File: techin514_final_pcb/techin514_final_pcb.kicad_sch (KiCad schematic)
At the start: 6 parts, among them M1 Motor_Servo, U1 ESP32-C3-DevKitM-1, U2 HC-SR04, U3 HC-SR04, U4 ESP32-C3-DevKitM-1

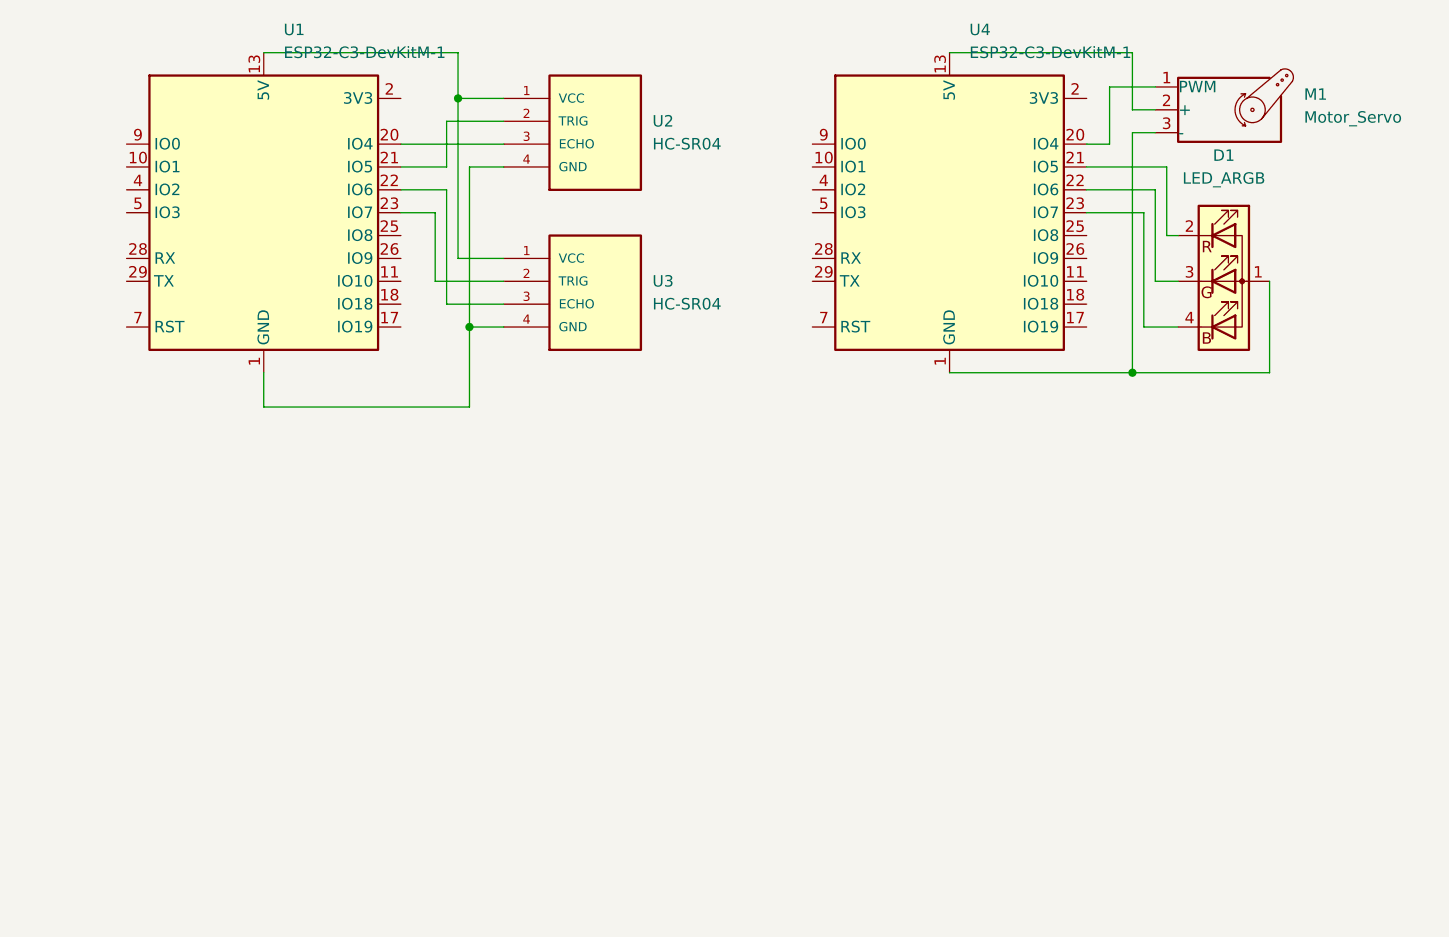
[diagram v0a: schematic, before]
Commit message: Datasheet updated
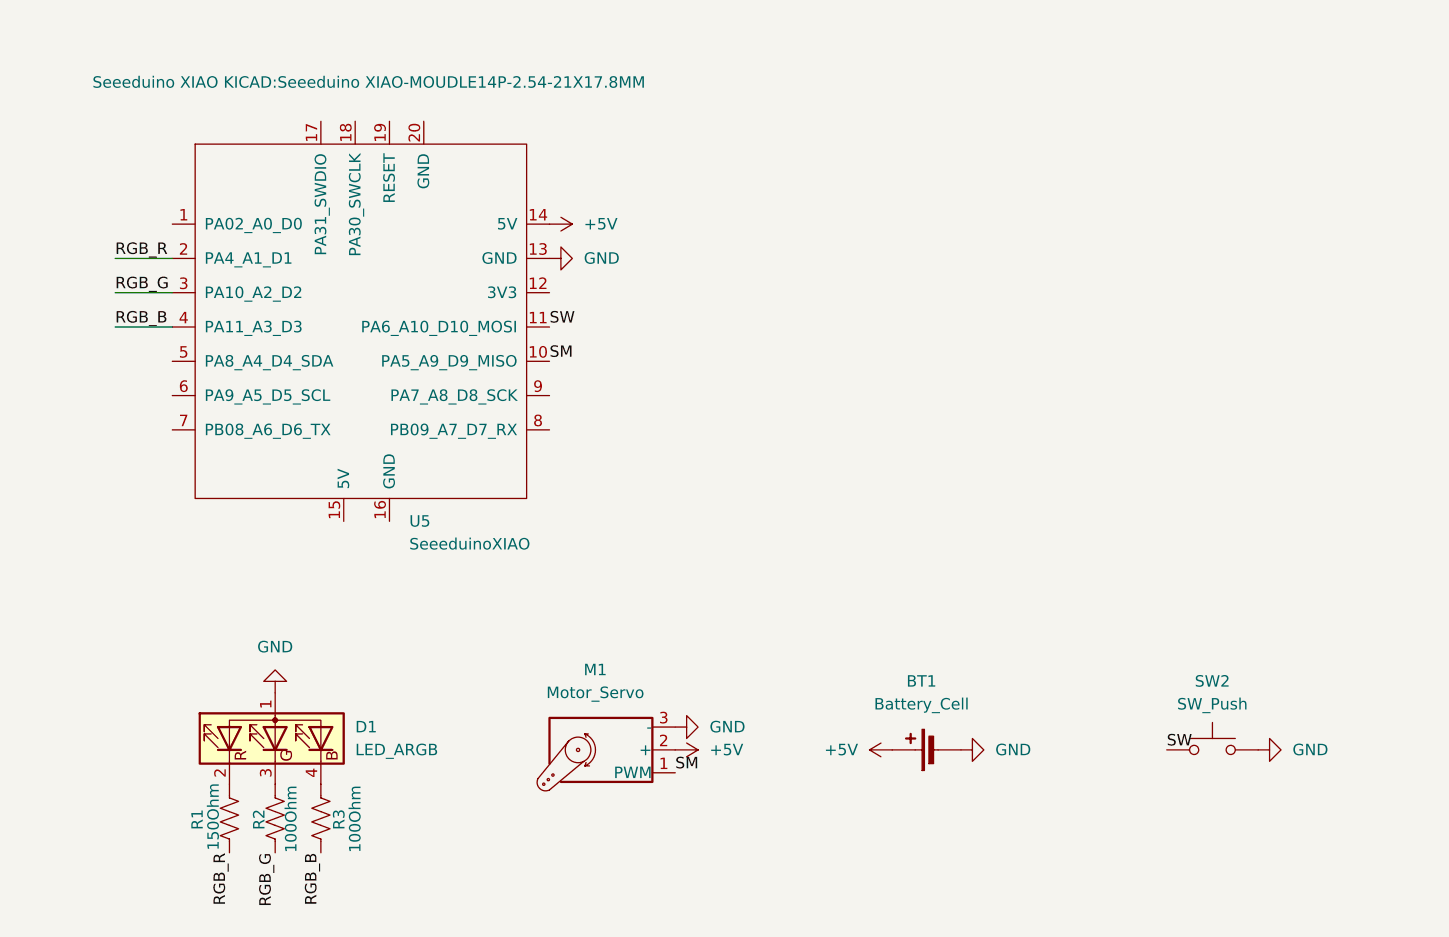
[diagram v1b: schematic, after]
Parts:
- removed U1, U4: ESP32-C3-DevKitM-1, RF_Module:ESP32-C3-DevKitM-1, symbol RF_Module:ESP32-C3-DevKitM-1
- removed U2, U3: HC-SR04, HC-SR04:XCVR_HC-SR04, symbol HC-SR04:HC-SR04
- added BT1: Battery_Cell, Connector_JST:JST_PH_B2B-PH-K_1x02_P2.00mm_Vertical, symbol Device:Battery_Cell
- added R1: 150Ohm, Resistor_SMD:R_0201_0603Metric, symbol Device:R_US
- added R2, R3: 100Ohm, Resistor_SMD:R_0201_0603Metric, symbol Device:R_US
- added SW2: SW_Push, Button_Switch_THT:SW_Tactile_Straight_KSA0Axx1LFTR, symbol Switch:SW_Push
- added U5: SeeeduinoXIAO, Seeeduino XIAO KICAD:Seeeduino XIAO-MOUDLE14P-2.54-21X17.8MM, symbol Seeeduino XIAO:SeeeduinoXIAO
- D1: footprint (none) -> LED_THT:LED_D5.0mm-4_RGB_Wide_Pins
- M1: footprint (none) -> Connector_PinHeader_2.54mm:PinHeader_1x03_P2.54mm_Vertical
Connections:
- net SM: now reaches M1.1 (PWM)
- net SM: now also U5.10 (PA5_A9_D9_MISO)
- net +5V: now reaches M1.2 (+)
- net +5V: now also BT1.1 (+), U5.14 (5V)
- net GND: now reaches D1.1 (A), M1.3 (-)
- net GND: now also BT1.2 (-), SW2.2, U5.13 (GND)
- net at D1.2 (RK): now also R1.1
- net at D1.3 (GK): now also R2.1
- net at D1.4 (BK): now also R3.1
- new net RGB_B: R3.2, U5.4 (PA11_A3_D3)
- new net RGB_G: R2.2, U5.3 (PA10_A2_D2)
- new net RGB_R: R1.2, U5.2 (PA4_A1_D1)
- new net SW: SW2.1, U5.11 (PA6_A10_D10_MOSI)
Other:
- company: (none) -> UW MSTI
- title: (none) -> Kyle
- moved on the sheet: D1, M1
